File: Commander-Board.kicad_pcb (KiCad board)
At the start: 2 copper layers, 99.1 x 99.1 mm, 26 parts, among them J1 POWER, J2 EXPAND, M1 3.5_TFT_SPI_480_320, SW1 BUTTON_BACK, SW2 BUTTON_ENTER, U1 AMS1117-3.3, U2 ACS711xLCTR-12AB, U3 ESP32-WROOM-32

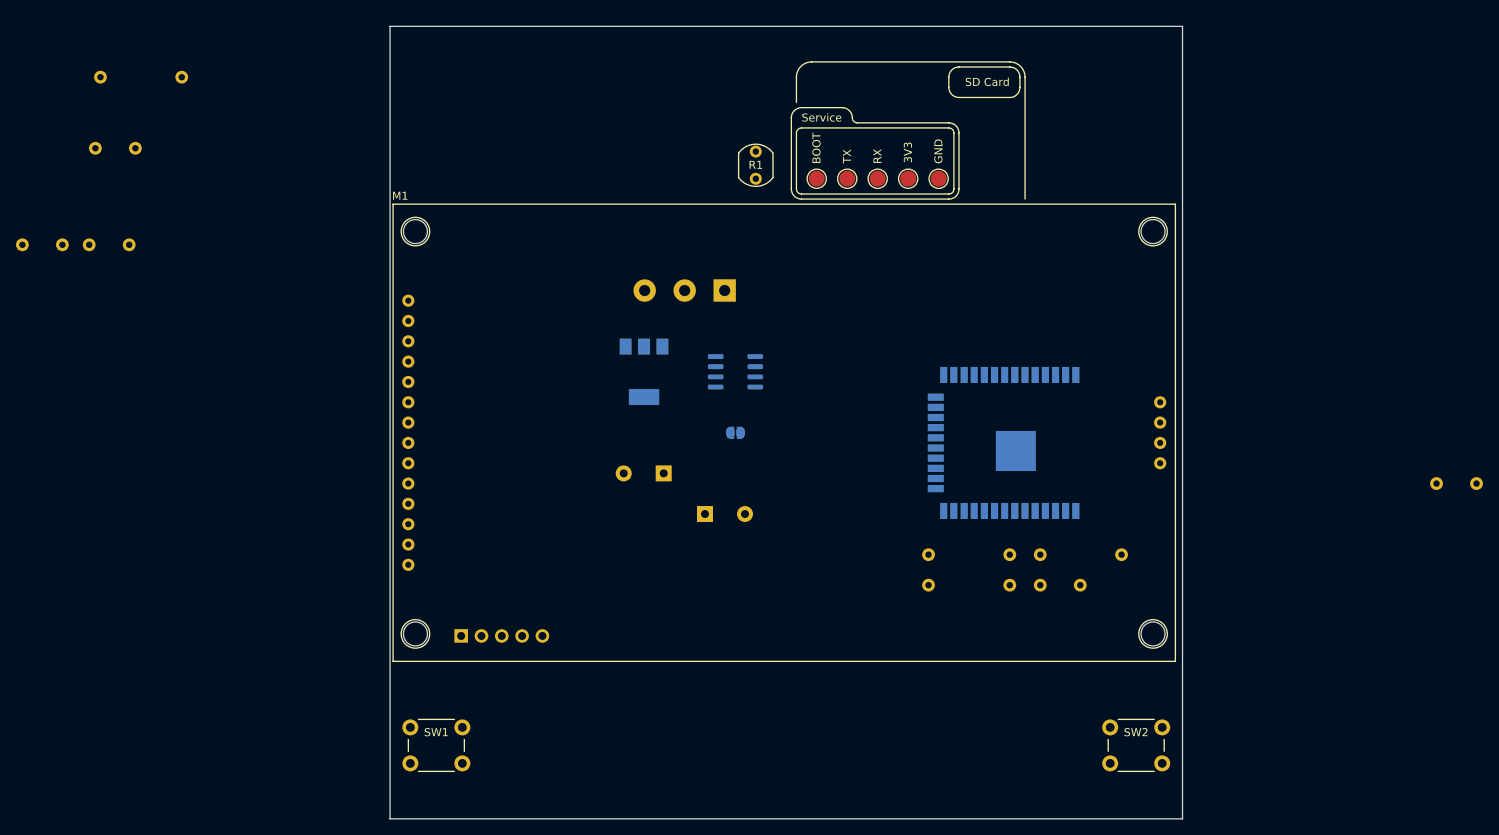
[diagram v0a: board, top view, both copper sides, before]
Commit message: Complete
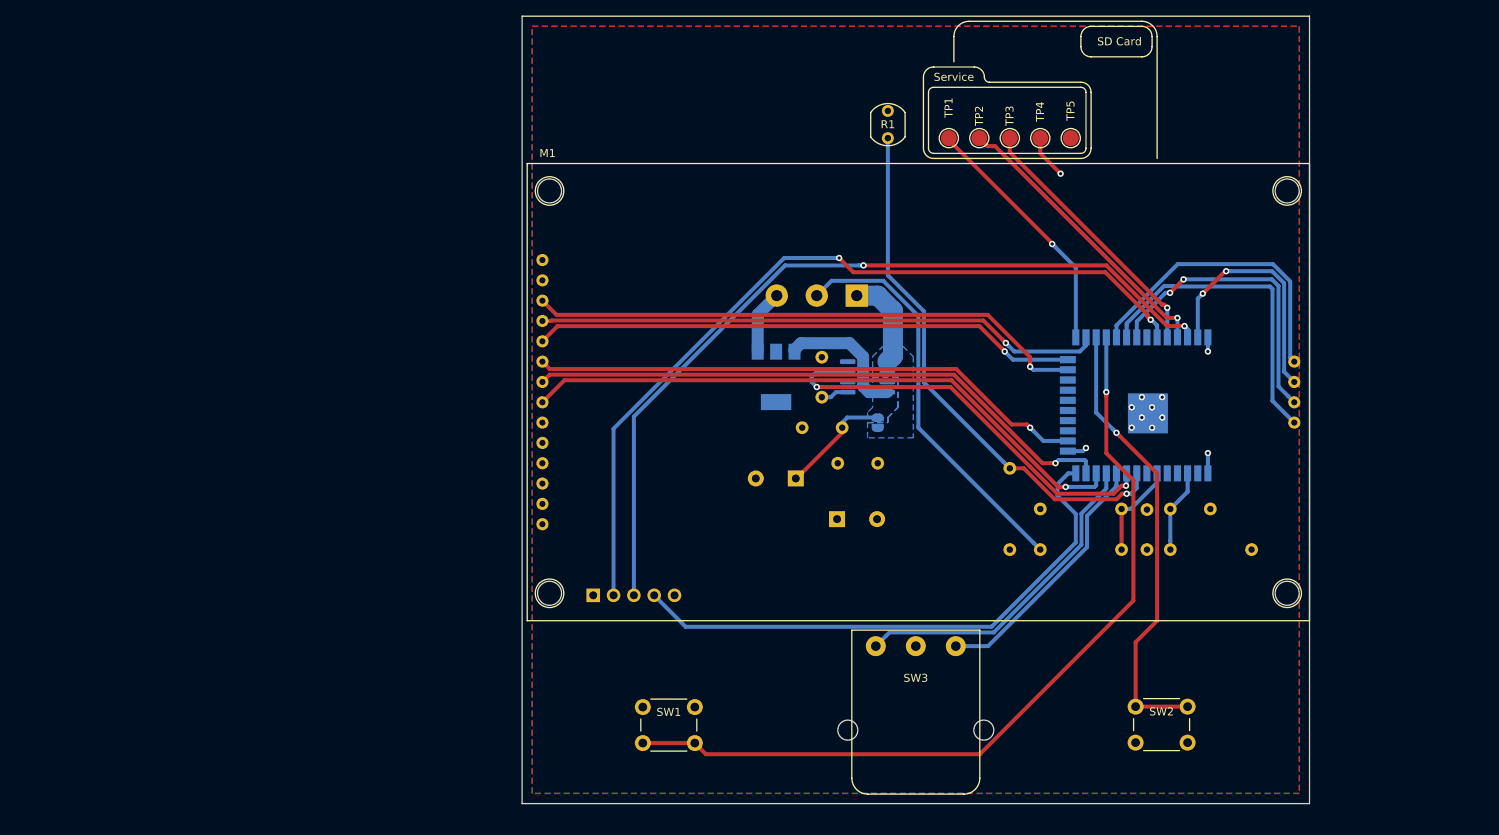
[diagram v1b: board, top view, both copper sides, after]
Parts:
- added SW3: Rotary_Encoder, ILI9488_Display:RotaryEncoder_Alps_EC16B04, F.Cu at (144.5, 129.5)
- moved C8 136.3 mm to (173.4, 112.5), turned to 270 degrees
- moved R2 114.5 mm to (156.2, 107.3), turned to 270 degrees
- moved C5 105.5 mm to (134.7, 106.7)
- moved C4 94.5 mm to (132.7, 93.4), turned to 270 degrees
- moved C3 74.6 mm to (135.3, 102.2), turned to 180 degrees
- moved SW1 29.2 mm to (110.3, 137.2)
- moved C9 18.8 mm to (181.3, 112.4)
- moved JP1 17.8 mm to (139.7, 101.6), turned to 270 degrees
- moved M1 17.5 mm to (95.9, 126.4)
- moved TP2 17.3 mm to (152.4, 66.0)
- moved TP3 17.3 mm to (156.2, 66.0)
- moved TP4 17.3 mm to (160.0, 66.0)
- moved TP5 17.3 mm to (163.8, 66.0)
- moved J2 17.3 mm to (104.1, 123.2)
- moved R1 17.3 mm to (141.0, 66.0)
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- renumbered BOOT to TP1, TX to TP2, RX to TP3, 3V3 to TP4, GND to TP5
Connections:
- M1 pad 1: (no net) -> Net-(M1-Pad1)
- M1 pad 10: (no net) -> /TFT_RS
- M1 pad 11: (no net) -> /TFT_RST
- M1 pad 12: (no net) -> /TFT_CS
- M1 pad 13: (no net) -> +3V3
- M1 pad 14: (no net) -> GND
- M1 pad 15: (no net) -> /SD_CS
- M1 pad 16: (no net) -> /SD_MOSI
- M1 pad 17: (no net) -> /SD_MISO
- M1 pad 18: (no net) -> /SD_SCK
- M1 pad 2: (no net) -> Net-(M1-Pad2)
- M1 pad 3: (no net) -> Net-(M1-Pad3)
- M1 pad 4: (no net) -> Net-(M1-Pad4)
- M1 pad 5: (no net) -> Net-(M1-Pad5)
- M1 pad 6: (no net) -> Net-(M1-Pad6)
- M1 pad 7: (no net) -> /TFT_BL
- M1 pad 8: (no net) -> /TFT_SCK
- M1 pad 9: (no net) -> /TFT_DI
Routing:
- net /PB_BACK: track 0.00 -> 104.2 mm, vias 0 -> 1
- net /EX_2: track 0.00 -> 103.7 mm, vias 0 -> 2
- net /EX_1: track 0.00 -> 102.8 mm, vias 0 -> 2
- net /TFT_BL: track 0.00 -> 77.5 mm, vias 0 -> 1
- net /TFT_SCK: track 0.00 -> 74.6 mm, vias 0 -> 1
- net /TFT_RST: track 0.00 -> 70.9 mm, vias 0 -> 1
- net /TFT_CS: track 0.00 -> 70.0 mm, vias 0 -> 1
- net /EX_3: track 0.00 -> 69.8 mm
- net /TFT_DI: track 0.00 -> 69.8 mm, vias 0 -> 1
- net /TFT_RS: track 0.00 -> 68.2 mm, vias 0 -> 1
- net /AN_LIGHT: track 0.00 -> 67.5 mm, vias 0 -> 1
- net /PB_ENT: track 0.00 -> 56.9 mm, vias 0 -> 1
- net /AN_CURR: track 0.00 -> 52.5 mm, vias 0 -> 2
- net Net-(J1-Pad2): track 0.00 -> 50.8 mm
- net /ENC_B: track 0.00 -> 41.2 mm
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- added copper zone on B.Cu, net +12V
- added copper zone on B.Cu, net +3V3
- added copper zone on F.Cu, net GND
- added copper zone on B.Cu, net Net-(J1-Pad1)
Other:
- board size 99.1 x 99.1 mm -> 98.4 x 98.4 mm
- board text added: "Power supply"
